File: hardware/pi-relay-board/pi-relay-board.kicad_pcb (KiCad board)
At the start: 2 copper layers, 44 parts, among them J1 Raspberry_Pi_2_3, J10 Conn_01x03_Socket, J11 Conn_01x03_Socket, J2 Conn_01x03_Socket, J3 Conn_01x03_Socket, J4 Conn_01x03_Socket, J5 Conn_01x03_Socket, J6 Conn_01x03_Socket, J7 Conn_01x03_Socket, J8 Conn_01x03_Socket, J9 Conn_01x03_Socket, K1 TIANBO-HJR-4102-L, K10 TIANBO-HJR-4102-L, K2 TIANBO-HJR-4102-L, K3 TIANBO-HJR-4102-L, K4 TIANBO-HJR-4102-L, K5 TIANBO-HJR-4102-L, K6 TIANBO-HJR-4102-L, K7 TIANBO-HJR-4102-L, K8 TIANBO-HJR-4102-L, K9 TIANBO-HJR-4102-L, Q1 BC547, Q10 BC547, Q2 BC547, Q3 BC547, Q4 BC547, Q5 BC547, Q6 BC547, Q7 BC547, Q8 BC547, Q9 BC547

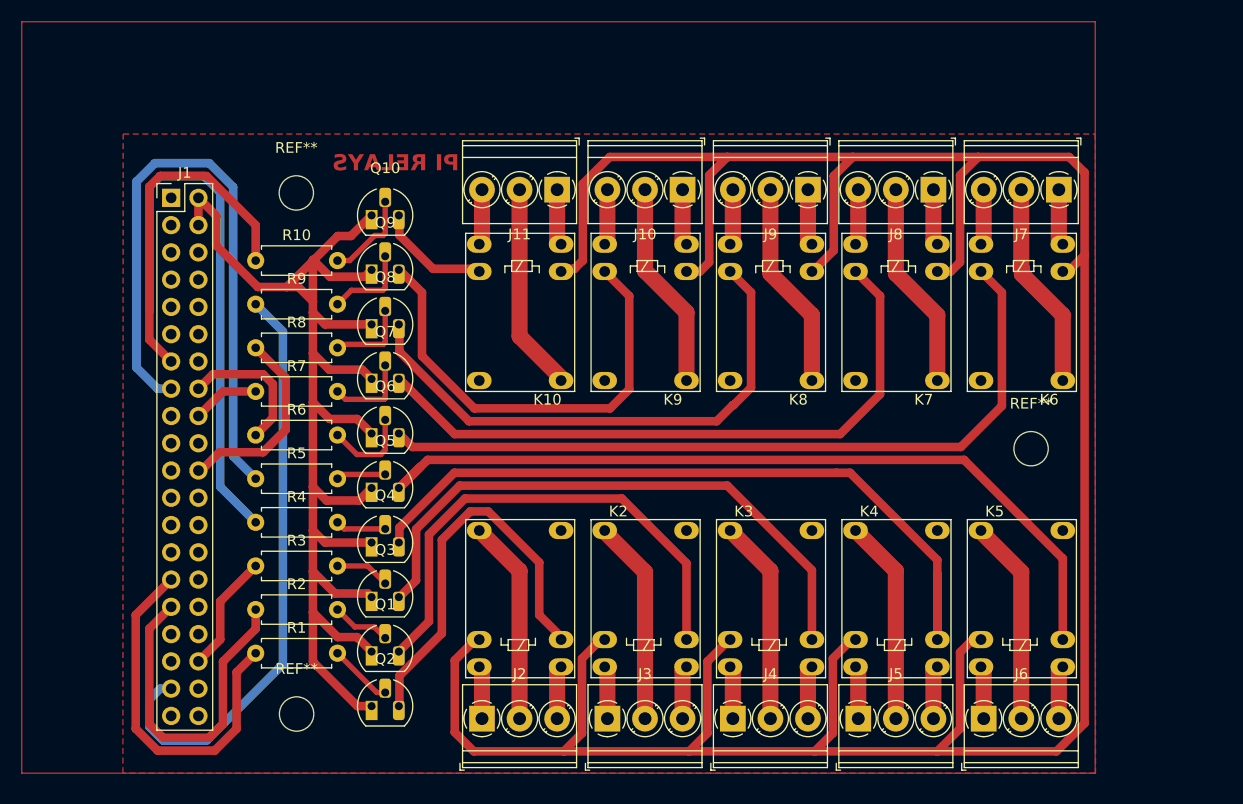
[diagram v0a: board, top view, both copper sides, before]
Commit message: fix: final finishes
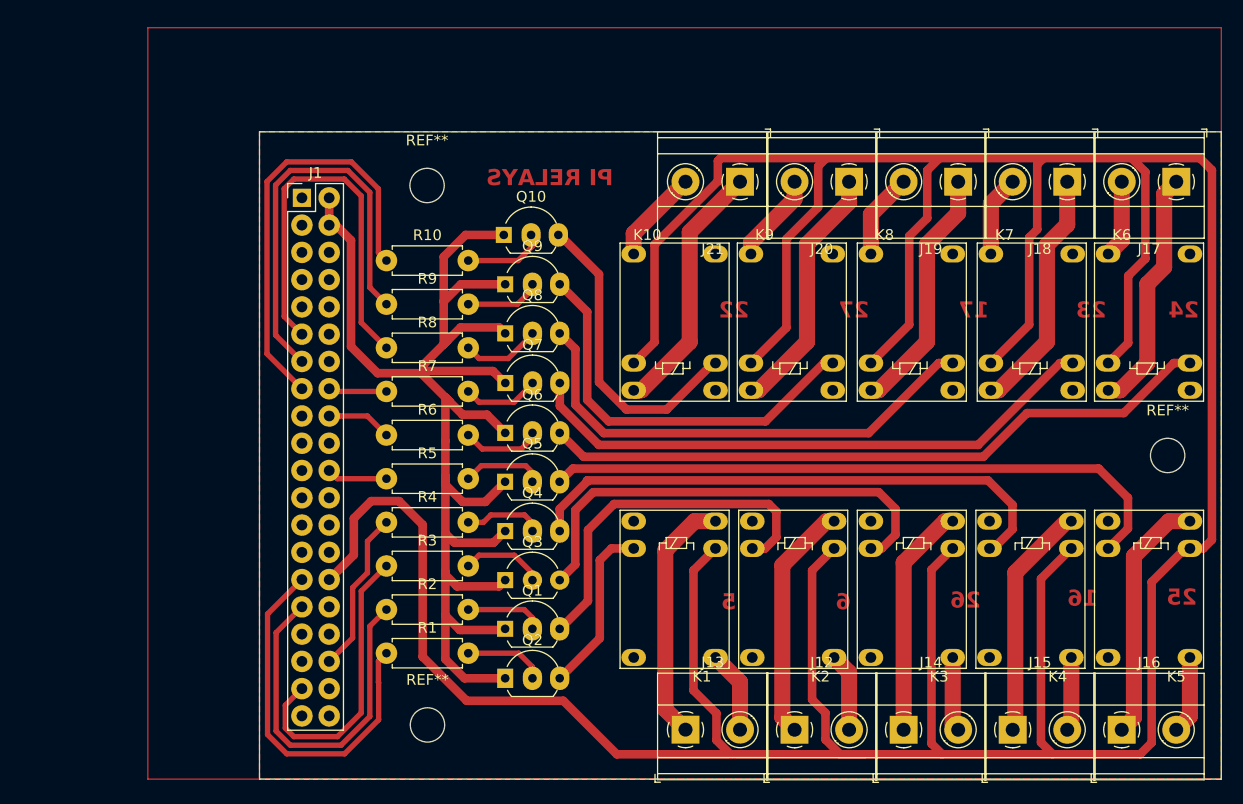
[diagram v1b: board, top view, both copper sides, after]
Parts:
- removed J10, J11, J2, J3, J4, J5, J6, J7, J8, J9: Conn_01x03_Socket, TerminalBlock_Phoenix:TerminalBlock_Phoenix_PT-1,5-3-3.5-H_1x03_P3.50mm_Horizontal
- added J12: Conn_01x02_Socket, TerminalBlock_Phoenix:TerminalBlock_Phoenix_MKDS-1,5-2-5.08_1x02_P5.08mm_Horizontal, F.Cu at (88.0, 81.4)
- added J13: Conn_01x02_Socket, TerminalBlock_Phoenix:TerminalBlock_Phoenix_MKDS-1,5-2-5.08_1x02_P5.08mm_Horizontal, F.Cu at (77.9, 81.4)
- added J14: Conn_01x02_Socket, TerminalBlock_Phoenix:TerminalBlock_Phoenix_MKDS-1,5-2-5.08_1x02_P5.08mm_Horizontal, F.Cu at (98.2, 81.4)
- added J15: Conn_01x02_Socket, TerminalBlock_Phoenix:TerminalBlock_Phoenix_MKDS-1,5-2-5.08_1x02_P5.08mm_Horizontal, F.Cu at (108.4, 81.4)
- added J16: Conn_01x02_Socket, TerminalBlock_Phoenix:TerminalBlock_Phoenix_MKDS-1,5-2-5.08_1x02_P5.08mm_Horizontal, F.Cu at (118.5, 81.4)
- added J17: Conn_01x02_Socket, TerminalBlock_Phoenix:TerminalBlock_Phoenix_MKDS-1,5-2-5.08_1x02_P5.08mm_Horizontal, F.Cu at (123.6, 30.3)
- added J18: Conn_01x02_Socket, TerminalBlock_Phoenix:TerminalBlock_Phoenix_MKDS-1,5-2-5.08_1x02_P5.08mm_Horizontal, F.Cu at (113.4, 30.3)
- added J19: Conn_01x02_Socket, TerminalBlock_Phoenix:TerminalBlock_Phoenix_MKDS-1,5-2-5.08_1x02_P5.08mm_Horizontal, F.Cu at (103.3, 30.3)
- added J20: Conn_01x02_Socket, TerminalBlock_Phoenix:TerminalBlock_Phoenix_MKDS-1,5-2-5.08_1x02_P5.08mm_Horizontal, F.Cu at (93.1, 30.3)
- added J21: Conn_01x02_Socket, TerminalBlock_Phoenix:TerminalBlock_Phoenix_MKDS-1,5-2-5.08_1x02_P5.08mm_Horizontal, F.Cu at (83.0, 30.3)
- Q1, Q10, Q2, Q3, Q4, Q5, Q6, Q7, Q8, Q9: footprint Package_TO_SOT_THT:TO-92_HandSolder -> Package_TO_SOT_THT:TO-92L_Inline_Wide
- moved K1 25.0 mm to (80.7, 74.7), turned to 180 degrees
- moved K2 24.4 mm to (91.7, 74.7), turned to 180 degrees
- moved K3 23.9 mm to (102.8, 74.7), turned to 180 degrees
- moved K4 23.3 mm to (113.8, 74.7), turned to 180 degrees
- moved K5 22.8 mm to (124.9, 74.7), turned to 180 degrees
- moved K10 13.6 mm to (73.1, 37.1), turned to 0 degrees
- moved K9 13.2 mm to (84.0, 37.1), turned to 0 degrees
- moved K8 13.0 mm to (95.2, 37.1), turned to 0 degrees
- moved K7 12.8 mm to (106.3, 37.1), turned to 0 degrees
- moved REF** 12.7 mm to (122.8, 55.9)
- moved Q2 12.7 mm to (61.1, 76.6)
- moved Q1 12.6 mm to (61.1, 72.0)
- moved Q3 12.5 mm to (61.1, 67.5)
- moved K6 12.5 mm to (117.3, 37.1), turned to 0 degrees
- moved Q9 12.5 mm to (61.1, 39.9)
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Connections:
- J1 pad 11: /Relay Pin 4/K -> /Relay Pin 8/K
- J1 pad 13: /Relay Pin 10/K -> /Relay Pin 9/K
- J1 pad 15: /Relay Pin 5/K -> /Relay Pin 10/K
- J1 pad 16: /Relay Pin 6/K -> /Relay Pin 7/K
- J1 pad 18: /Relay Pin 7/K -> /Relay Pin 6/K
- J1 pad 22: /Relay Pin 8/K -> /Relay Pin 5/K
- J1 pad 36: /GPIO16 -> /Relay Pin 4/K
- J1 pad 37: /Relay Pin 9/K -> /Relay Pin 3/K
- K1 pad 7: Net-(J2-Pin_3) -> unconnected-(K1-Pad7)
- K10 pad 7: Net-(J11-Pin_3) -> unconnected-(K10-Pad7)
- K2 pad 7: Net-(J3-Pin_3) -> unconnected-(K2-Pad7)
- K3 pad 7: Net-(J4-Pin_3) -> unconnected-(K3-Pad7)
- K4 pad 7: Net-(J5-Pin_3) -> unconnected-(K4-Pad7)
- K5 pad 7: Net-(J6-Pin_3) -> unconnected-(K5-Pad7)
- K6 pad 7: Net-(J7-Pin_3) -> unconnected-(K6-Pad7)
- K7 pad 7: Net-(J8-Pin_3) -> unconnected-(K7-Pad7)
- K8 pad 7: Net-(J9-Pin_3) -> unconnected-(K8-Pad7)
- K9 pad 7: Net-(J10-Pin_3) -> unconnected-(K9-Pad7)
- R3 pad 1: /GPIO16 -> /Relay Pin 3/K
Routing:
- net GND: track 269.3 -> 397.5 mm
- net /Relay Pin 5/K: track 60.1 -> 5.90 mm
- net /Relay Pin 4/K: track 51.4 -> 15.2 mm
- net /Relay Pin 3/K: track 0.00 -> 28.0 mm
- net Net-(Q2-E): track 37.2 -> 16.2 mm
- net /Relay Pin 8/K: track 18.5 -> 37.6 mm
- net Net-(Q4-E): track 70.5 -> 51.5 mm
- net Net-(J21-Pin_1): track 5.23 -> 23.9 mm
- net Net-(J20-Pin_1): track 5.23 -> 23.6 mm
- net Net-(J13-Pin_1): track 4.93 -> 23.3 mm
- net Net-(Q10-E): track 10.6 -> 28.9 mm
- net Net-(J16-Pin_1): track 4.93 -> 23.2 mm
- net Net-(J18-Pin_1): track 5.23 -> 23.3 mm
- net Net-(J19-Pin_1): track 5.23 -> 23.2 mm
- net Net-(J17-Pin_1): track 5.23 -> 22.7 mm
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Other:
- board outline added: 89.6 x 60.3 mm
- board text added: "16"
- board text added: "17"
- board text added: "22"
- board text added: "23"
- board text added: "24"
- board text added: "25"
- board text added: "26"
- board text added: "27"
- board text added: "5"
- board text added: "6"
- board text added: "GPIO 16"
- board text added: "GPIO 17"
- board text added: "GPIO 22"
- board text added: "GPIO 23"
- board text added: "GPIO 24"
- board text added: "GPIO 25"
- board text added: "GPIO 26"
- board text added: "GPIO 27"
- board text added: "GPIO 5"
- board text added: "GPIO 6"
